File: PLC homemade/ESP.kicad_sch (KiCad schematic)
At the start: 9 parts, among them J6 1803316, U9 ESP32-S3-WROOM-1U-N16R8

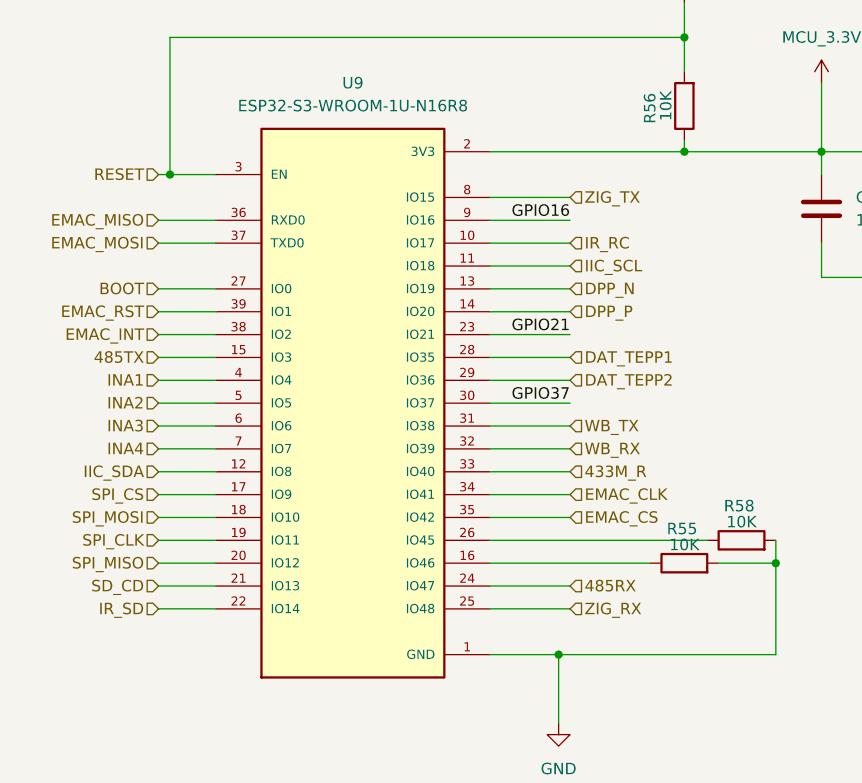
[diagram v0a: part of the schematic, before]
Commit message: :clown_face: changed HEIRACHIAL to global
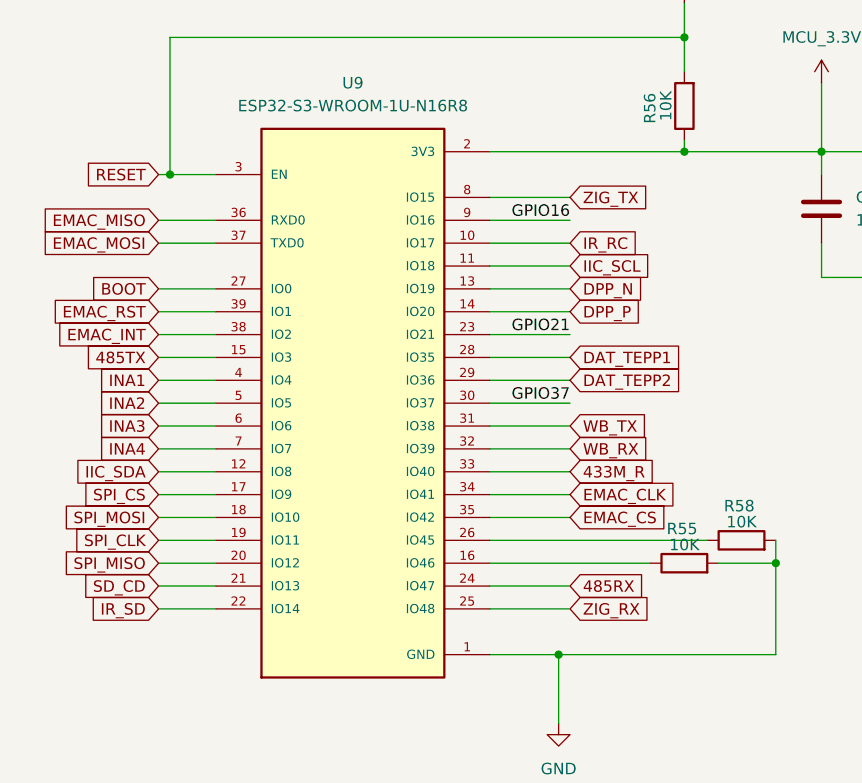
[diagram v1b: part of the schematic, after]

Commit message: :tada: Run Electrical rule checker All errors corrected
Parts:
- C34: footprint (none) -> Capacitor_SMD:C_01005_0402Metric
- C35, C36: footprint (none) -> Capacitor_SMD:C_0201_0603Metric
- R55, R56, R58: footprint (none) -> Resistor_SMD:R_01005_0402Metric
- R57: footprint (none) -> Resistor_SMD:R_0402_1005Metric
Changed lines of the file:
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@@
 			)
 		)
-		(property "Footprint" ""
+		(property "Footprint" "Resistor_SMD:R_0402_1005Metric"
 			(at 212.09 55.118 90)
 			(effects
@@
 			)
 		)
-		(property "Footprint" ""
+		(property "Footprint" "Resistor_SMD:R_01005_0402Metric"
 			(at 168.91 98.298 90)
 			(effects
@@
 			)
 		)
-		(property "Footprint" ""
+		(property "Footprint" "Capacitor_SMD:C_01005_0402Metric"
 			(at 178.7652 63.5 0)
 			(effects
@@
 			)
 		)
-		(property "Footprint" ""
+		(property "Footprint" "Capacitor_SMD:C_0201_0603Metric"
 			(at 163.5252 36.83 0)
 			(effects
@@
 			)
 		)
-		(property "Footprint" ""
+		(property "Footprint" "Capacitor_SMD:C_0201_0603Metric"
 			(at 196.5452 63.5 0)
 			(effects
@@
 			)
 		)
-		(property "Footprint" ""
+		(property "Footprint" "Resistor_SMD:R_01005_0402Metric"
 			(at 164.338 48.26 90)
 			(effects
@@
 			)
 		)
-		(property "Footprint" ""
+		(property "Footprint" "Resistor_SMD:R_01005_0402Metric"
 			(at 162.56 100.838 90)
 			(effects
